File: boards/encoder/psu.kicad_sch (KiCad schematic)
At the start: 10 parts, among them J6 PWR, U10 TPS62A02A

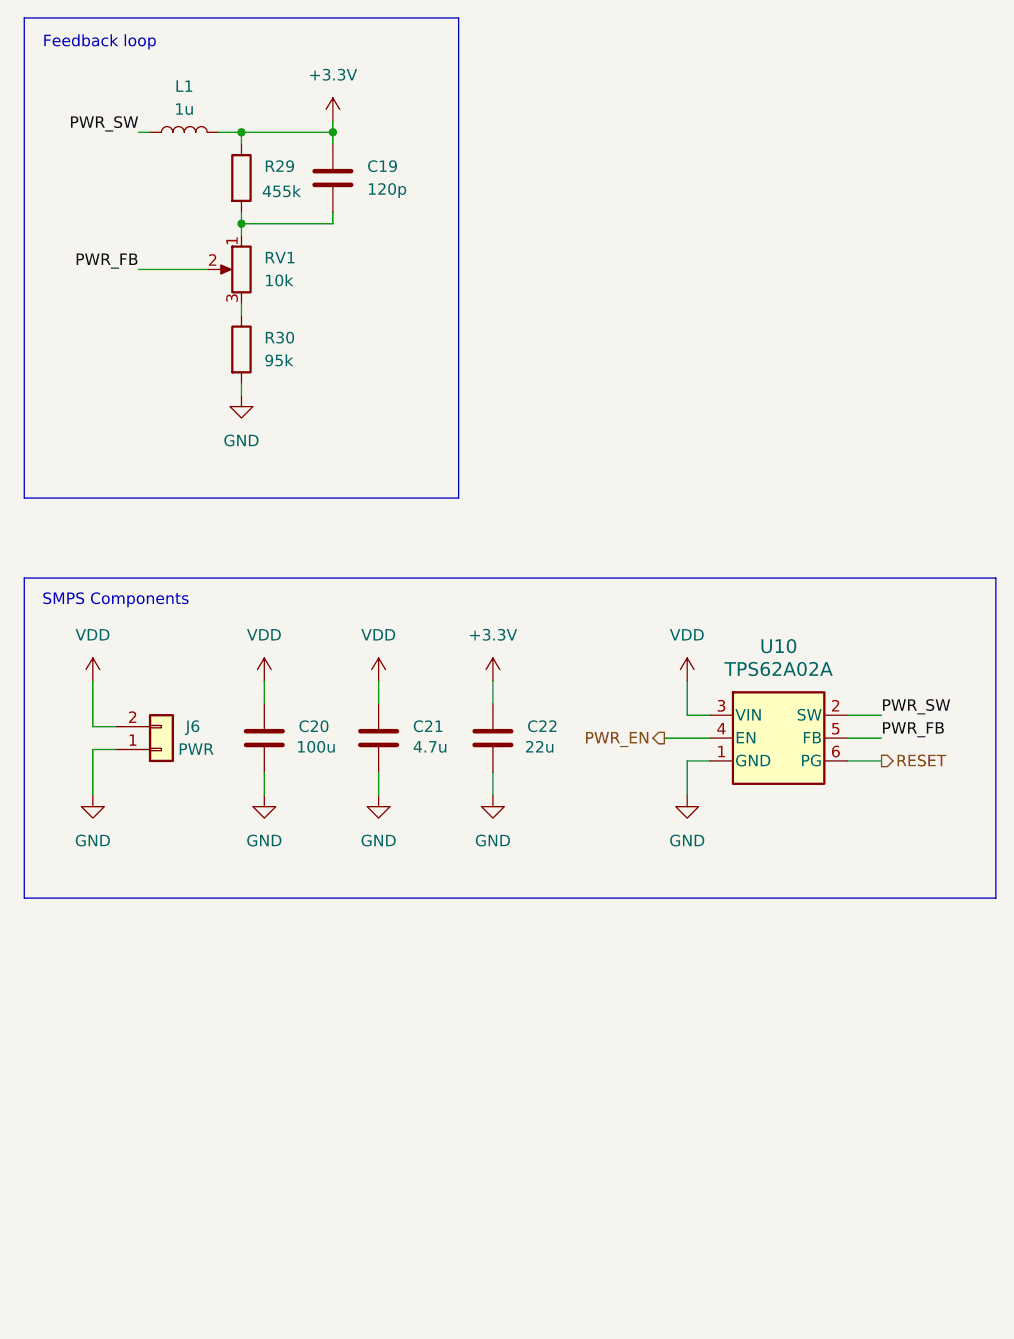
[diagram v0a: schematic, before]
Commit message: v0.3.6
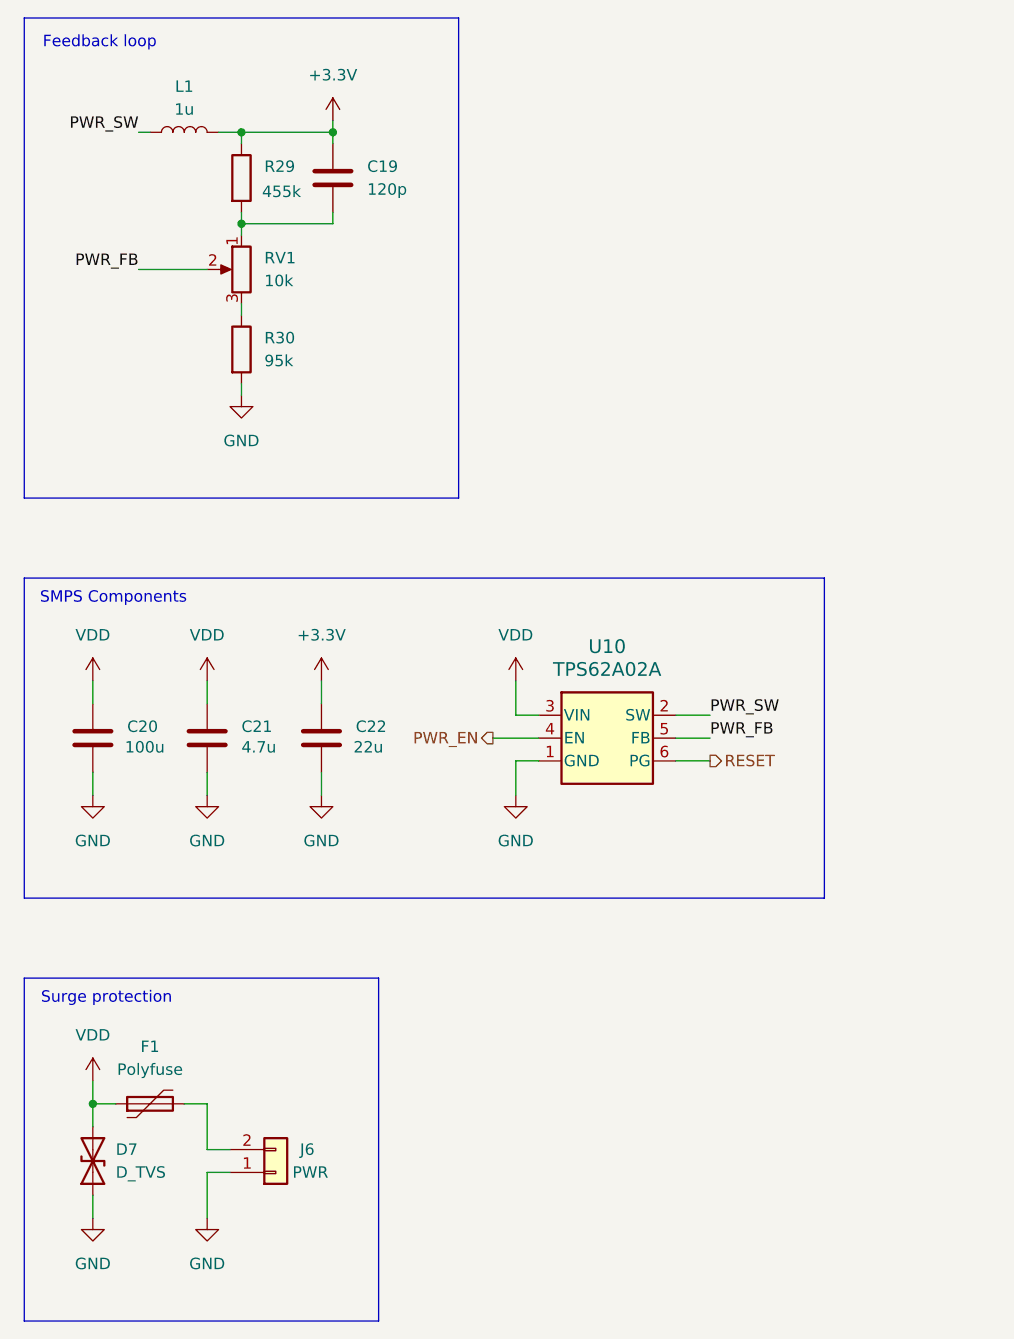
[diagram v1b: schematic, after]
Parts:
- added D7: D_TVS, Diode_SMD:D_SOD-523, symbol Device:D_TVS
- added F1: Polyfuse, Fuse:Fuse_1206_3216Metric, symbol Device:Polyfuse
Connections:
- net GND: now also D7.1 (A1)
- net VDD: now also D7.2 (A2), F1.1; no longer J6.2 (Pin_2)
- new net: F1.2, J6.2 (Pin_2)
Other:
- note added: "Surge protection"
- moved on the sheet: C20, C21, C22, J6, U10
